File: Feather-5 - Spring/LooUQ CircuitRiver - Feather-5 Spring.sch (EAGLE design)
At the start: 11 parts, among them J1 FEATHERHOST-S, J2 FEATHERHOST-L, J3 CR-SPRING_HEADER, J4 JST_PH-2_T/H, J5 JST_PH-2_T/H, J6 QWIIC_VERTICAL, J7 CR-RAPIDSIO_VERTICAL, J8 DNF, P3 SLEEP

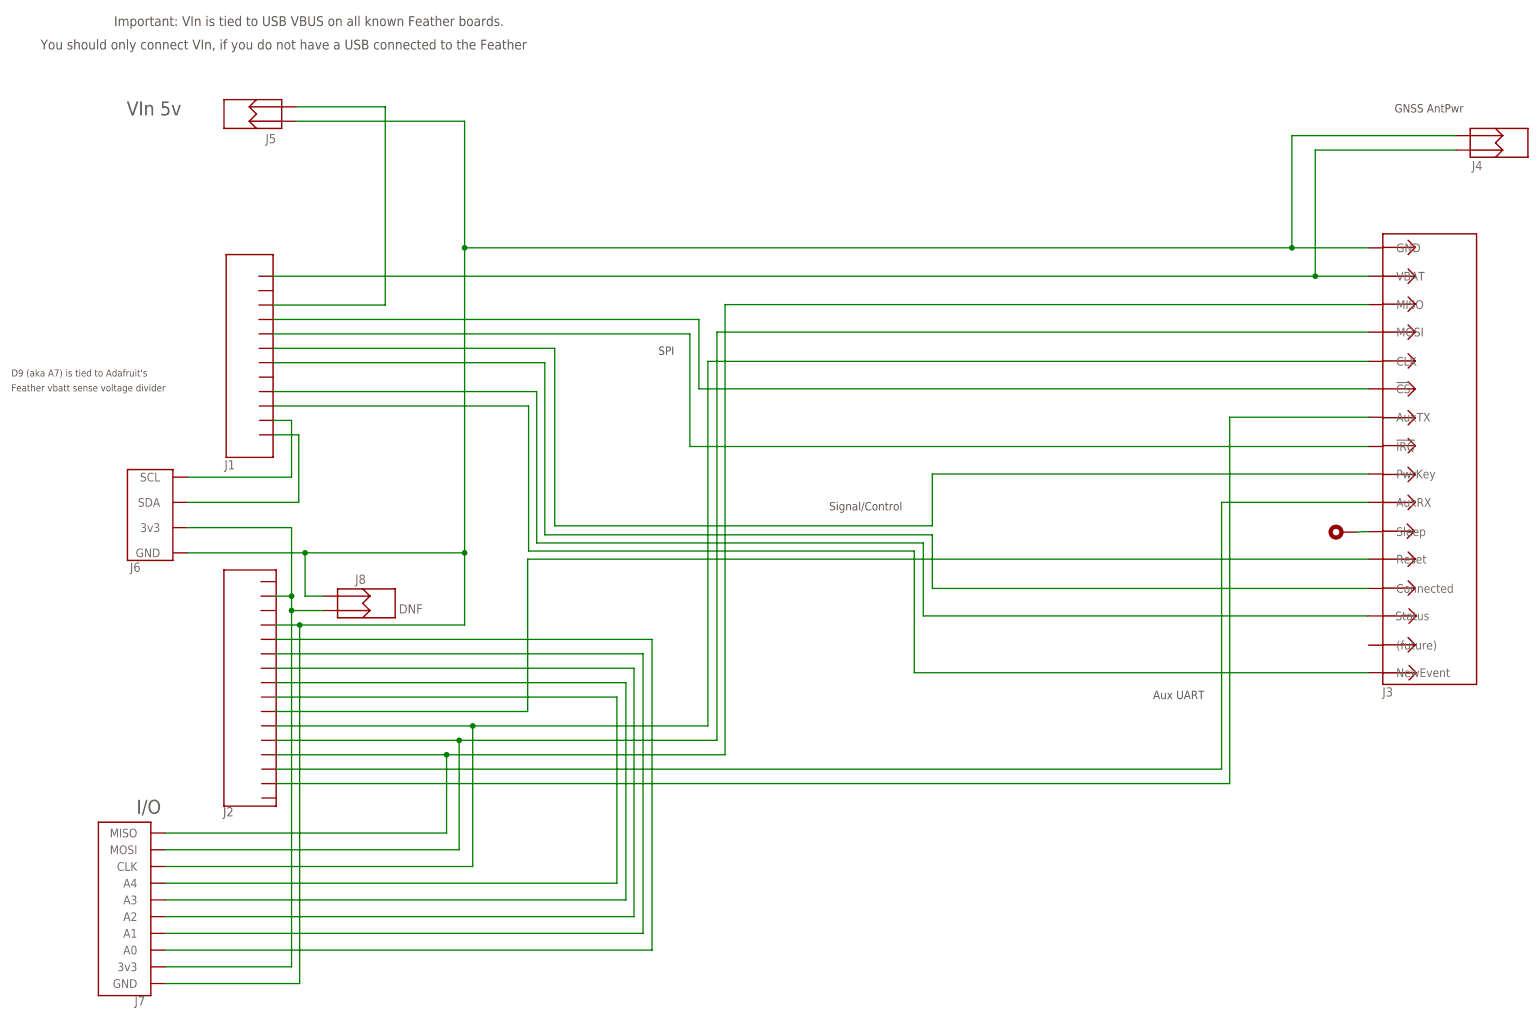
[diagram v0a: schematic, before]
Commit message: Updated Feathers
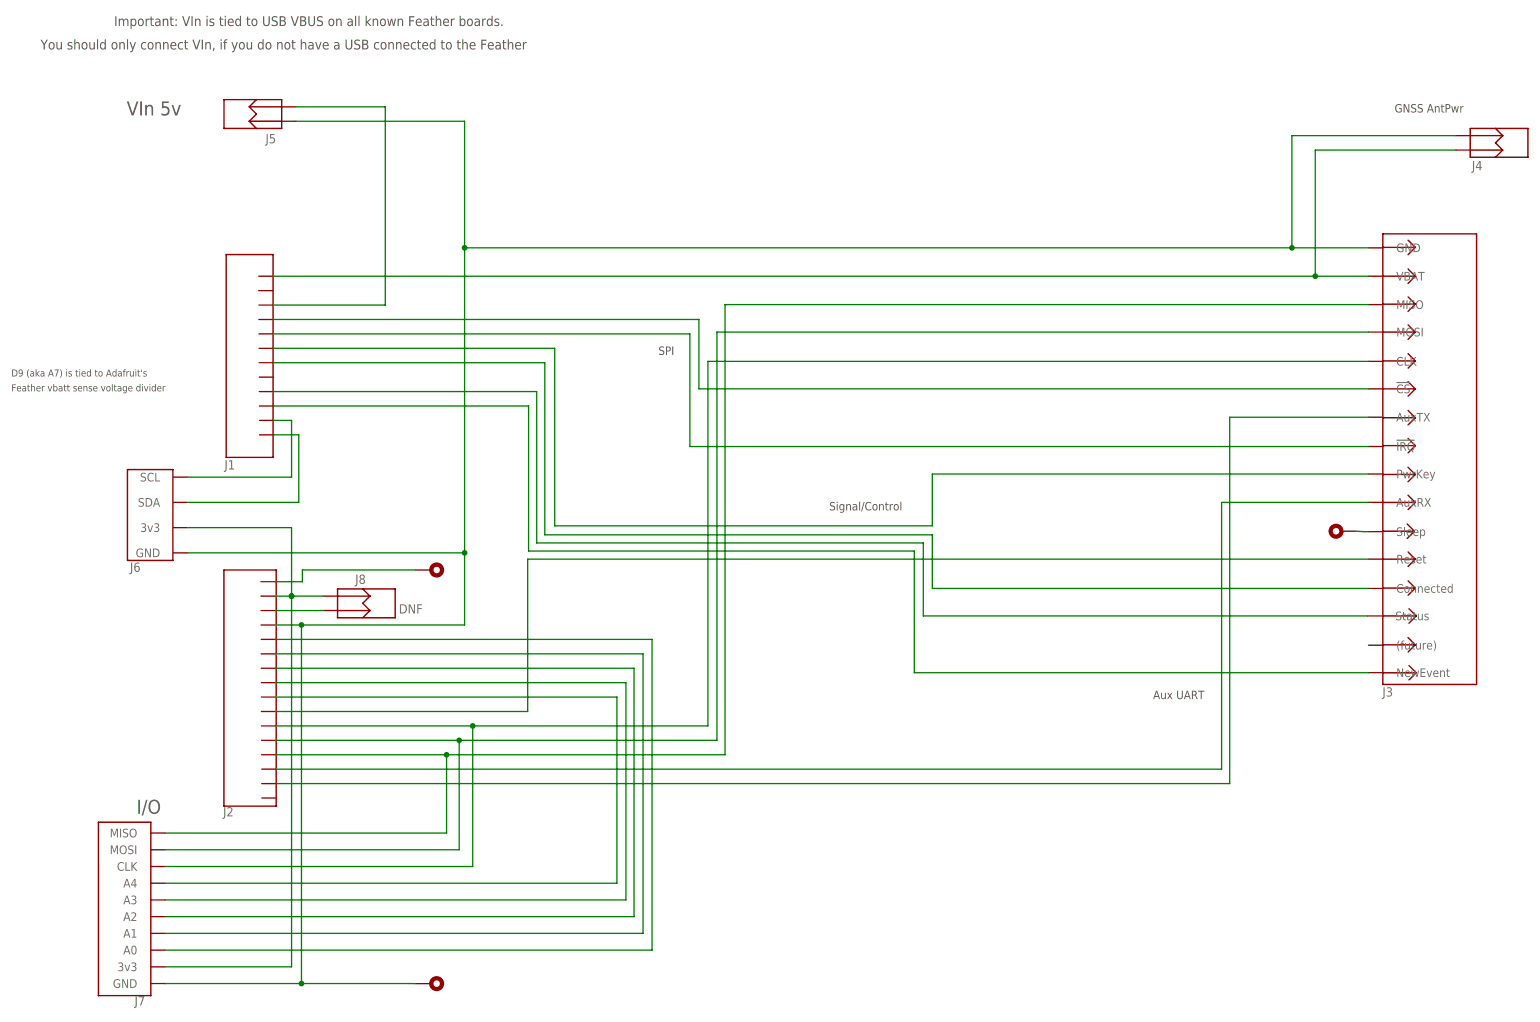
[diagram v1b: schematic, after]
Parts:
- added P1: DNF, common:~RESET
- added P2: DNF, common:GND
- P3: value SLEEP -> DNF
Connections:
- new net Net_0: J2.!RESET, P1.1
- new net Net_24: J2.AREF, J8.P1
- net Net_3v3: now also J8.P2; no longer J8.P1
- net Net_GND: now also P2.1; no longer J8.P2
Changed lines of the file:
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@@
 <part name="LG1" library="common" deviceset="LOOUQ_LOGO" device=""/>
 <part name="LG2" library="common" deviceset="CIRCUITRIVER_LOGO" device=""/>
-<part name="P3" library="common" deviceset="SLEEP" device=""/>
+<part name="P1" library="common" deviceset="~RESET" device="" value="DNF"/>
+<part name="P2" library="common" deviceset="GND" device="" value="DNF"/>
+<part name="P3" library="common" deviceset="SLEEP" device="" value="DNF"/>
 </parts>
 <modules/>
@@
 <instance part="LG1" gate="PART_1" x="91.122" y="86.995"/>
 <instance part="LG2" gate="PART_1" x="91.587" y="80.96"/>
-<instance part="P3" gate="BRKOUTPAD" x="101.362" y="-6.033" rot="R270"/>
+<instance part="P1" gate="BRKOUTPAD" x="-57.229" y="-12.7" rot="R90"/>
+<instance part="P2" gate="BRKOUTPAD" x="-57.229" y="-85.566" rot="R90"/>
+<instance part="P3" gate="BRKOUTPAD" x="101.362" y="-5.874" rot="R270"/>
 </instances>
 <busses/>
@@
 <net name="Net_22" class="0">
 <segment>
-<wire layer="91" width="0.25" x1="106.204" y1="-5.95" x2="104.934" y2="-6.033"/>
+<wire layer="91" width="0.25" x1="106.204" y1="-5.95" x2="104.934" y2="-5.874"/>
 <wire layer="91" width="0.25" x1="106.204" y1="-5.95" x2="106.986" y2="-5.95"/>
 <pinref part="P3" gate="BRKOUTPAD" pin="1"/>
@@
 <net name="Net_3v3" class="1">
 <segment>
-<wire layer="91" width="0.25" x1="-77.153" y1="-19.844" x2="-82.709" y2="-19.844"/>
-<wire layer="91" width="0.25" x1="-82.709" y1="-19.844" x2="-82.709" y2="-17.308"/>
-<wire layer="91" width="0.25" x1="-82.709" y1="-17.308" x2="-85.563" y2="-17.308"/>
-<pinref part="J8" gate="PART_1" pin="P1"/>
-<pinref part="J2" gate="PART_1" pin="+3V3"/>
 <wire layer="91" width="0.25" x1="-100.965" y1="-5.239" x2="-82.709" y2="-5.239"/>
 <wire layer="91" width="0.25" x1="-82.709" y1="-5.239" x2="-82.709" y2="-17.308"/>
+<wire layer="91" width="0.25" x1="-82.709" y1="-17.308" x2="-82.709" y2="-17.304"/>
+<wire layer="91" width="0.25" x1="-82.709" y1="-17.304" x2="-82.709" y2="-82.605"/>
+<wire layer="91" width="0.25" x1="-82.709" y1="-82.605" x2="-104.989" y2="-82.605"/>
 <pinref part="J6" gate="PART_1" pin="3v3"/>
+<pinref part="J7" gate="PART_1" pin="3v3"/>
+<wire layer="91" width="0.25" x1="-77.153" y1="-17.304" x2="-82.709" y2="-17.304"/>
+<pinref part="J8" gate="PART_1" pin="P2"/>
+<junction x="-82.709" y="-17.304"/>
+<wire layer="91" width="0.25" x1="-85.563" y1="-17.308" x2="-82.709" y2="-17.308"/>
+<pinref part="J2" gate="PART_1" pin="+3V3"/>
 <junction x="-82.709" y="-17.308"/>
-<wire layer="91" width="0.25" x1="-82.709" y1="-19.844" x2="-82.709" y2="-82.605"/>
-<wire layer="91" width="0.25" x1="-82.709" y1="-82.605" x2="-104.989" y2="-82.605"/>
-<pinref part="J7" gate="PART_1" pin="3v3"/>
-<junction x="-82.709" y="-19.844"/>
 </segment>
 </net>
 <net name="Net_GND" class="1">
 <segment>
-<wire layer="91" width="0.25" x1="-85.542" y1="-22.388" x2="-81.28" y2="-22.388"/>
-<wire layer="91" width="0.25" x1="-81.28" y1="-22.388" x2="-52.229" y2="-22.388"/>
+<wire layer="91" width="0.25" x1="-85.542" y1="-22.388" x2="-80.962" y2="-22.388"/>
+<wire layer="91" width="0.25" x1="-80.962" y1="-22.388" x2="-52.229" y2="-22.388"/>
 <wire layer="91" width="0.25" x1="-52.229" y1="-22.388" x2="-52.229" y2="-9.684"/>
 <wire layer="91" width="0.25" x1="-52.229" y1="-9.684" x2="-52.229" y2="44.05"/>
@@
 <pinref part="J5" gate="PART_1" pin="P2"/>
 <junction x="-52.229" y="44.05"/>
-<wire layer="91" width="0.25" x1="-100.965" y1="-9.684" x2="-80.327" y2="-9.684"/>
-<wire layer="91" width="0.25" x1="-80.327" y1="-9.684" x2="-52.229" y2="-9.684"/>
+<wire layer="91" width="0.25" x1="-100.965" y1="-9.684" x2="-52.229" y2="-9.684"/>
 <pinref part="J6" gate="PART_1" pin="GND"/>
 <junction x="-52.229" y="-9.684"/>
-<wire layer="91" width="0.25" x1="-77.153" y1="-17.304" x2="-80.327" y2="-17.304"/>
-<wire layer="91" width="0.25" x1="-80.327" y1="-17.304" x2="-80.327" y2="-9.684"/>
-<pinref part="J8" gate="PART_1" pin="P2"/>
-<junction x="-80.327" y="-9.684"/>
-<wire layer="91" width="0.25" x1="-81.28" y1="-22.388" x2="-81.28" y2="-85.551"/>
-<wire layer="91" width="0.25" x1="-81.28" y1="-85.551" x2="-104.989" y2="-85.551"/>
+<wire layer="91" width="0.25" x1="-80.962" y1="-22.388" x2="-80.962" y2="-85.551"/>
+<wire layer="91" width="0.25" x1="-80.962" y1="-85.551" x2="-104.989" y2="-85.551"/>
 <pinref part="J7" gate="PART_1" pin="GND"/>
-<junction x="-81.28" y="-22.388"/>
+<junction x="-80.962" y="-22.388"/>
+<wire layer="91" width="0.25" x1="-62.071" y1="-85.551" x2="-60.801" y2="-85.566"/>
+<wire layer="91" width="0.25" x1="-62.071" y1="-85.551" x2="-80.962" y2="-85.551"/>
+<pinref part="P2" gate="BRKOUTPAD" pin="1"/>
+<junction x="-80.962" y="-85.551"/>
 </segment>
 </net>
@@
 </segment>
 </net>
+<net name="Net_24" class="0">
+<segment>
+<wire layer="91" width="0.25" x1="-78.423" y1="-19.848" x2="-77.153" y2="-19.844"/>
+<wire layer="91" width="0.25" x1="-78.423" y1="-19.848" x2="-85.552" y2="-19.848"/>
+<pinref part="J8" gate="PART_1" pin="P1"/>
+<pinref part="J2" gate="PART_1" pin="AREF"/>
+</segment>
+</net>
+<net name="Net_0" class="0">
+<segment>
+<wire layer="91" width="0.25" x1="-60.801" y1="-12.7" x2="-80.804" y2="-12.7"/>
+<wire layer="91" width="0.25" x1="-80.804" y1="-12.7" x2="-80.804" y2="-14.768"/>
+<wire layer="91" width="0.25" x1="-80.804" y1="-14.768" x2="-85.573" y2="-14.768"/>
+<pinref part="P1" gate="BRKOUTPAD" pin="1"/>
+<pinref part="J2" gate="PART_1" pin="!RESET"/>
+</segment>
+</net>
